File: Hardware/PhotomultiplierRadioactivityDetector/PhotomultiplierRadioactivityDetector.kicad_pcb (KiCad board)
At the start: 2 copper layers, 100 x 100 mm, 102 parts, among them J13 Conn_01x02_Female, J14 Conn_01x04, J15 Conn_02x05_Counter_Clockwise, Q1 2N7002, Q2 Q_NPN_BEC, Q3 Q_NMOS_GDS, U1 TL074, U2 TL074, U3 MCP3425A0T-ECH, U4 LM3488, U5 STM8S003F3P

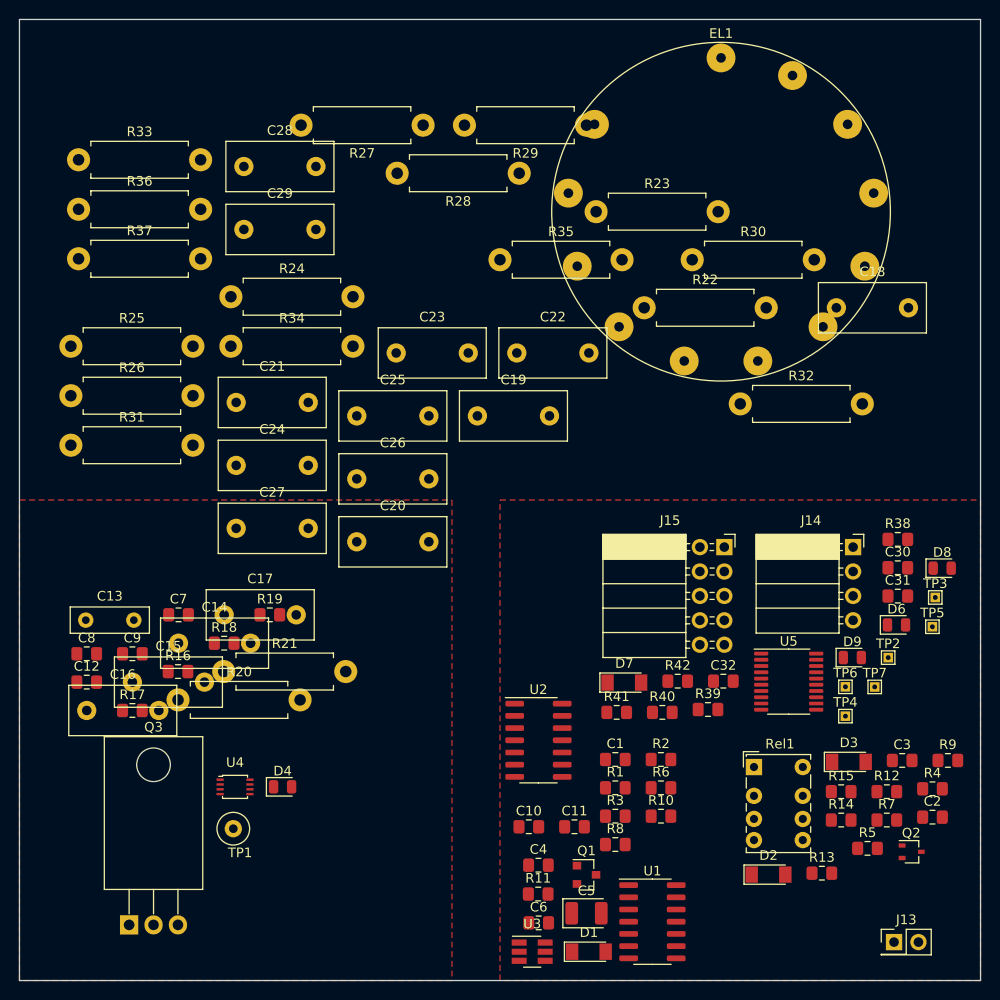
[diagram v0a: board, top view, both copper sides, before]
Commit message: draft of amplifier
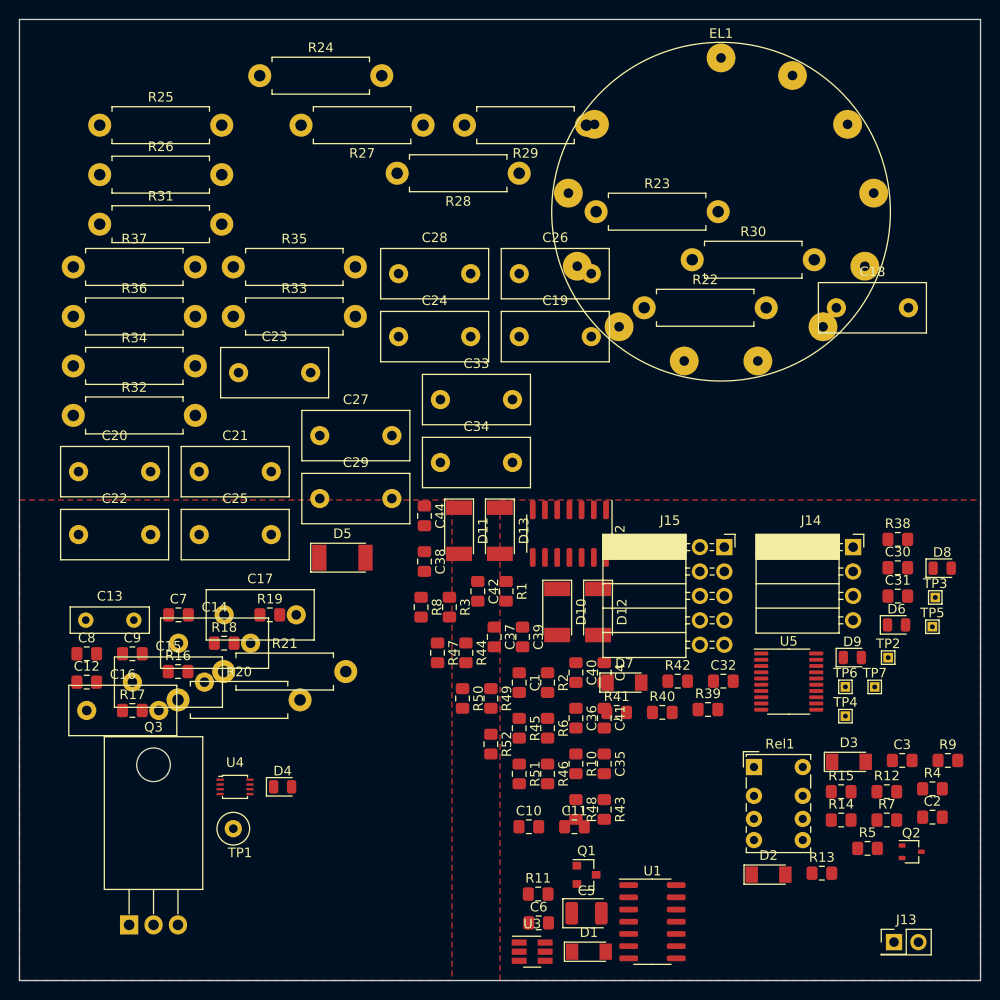
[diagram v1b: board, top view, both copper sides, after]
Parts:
- added C33: 10n/3kV, Capacitor_THT:C_Disc_D11.0mm_W5.0mm_P7.50mm, F.Cu at (68.8, 129.6)
- added C34: 10n/3kV, Capacitor_THT:C_Disc_D11.0mm_W5.0mm_P7.50mm, F.Cu at (68.8, 136.1)
- added C35: 2p2, Capacitor_SMD:C_0805_2012Metric_Pad1.15x1.40mm_HandSolder, F.Cu at (85.8, 167.4)
- added C36: 2p2, Capacitor_SMD:C_0805_2012Metric_Pad1.15x1.40mm_HandSolder, F.Cu at (82.9, 162.7)
- added C37: 1n, Capacitor_SMD:C_0805_2012Metric_Pad1.15x1.40mm_HandSolder, F.Cu at (74.4, 154.2)
- added C38: 1n, Capacitor_SMD:C_0805_2012Metric_Pad1.15x1.40mm_HandSolder, F.Cu at (67.1, 146.4)
- added C39: 100n, Capacitor_SMD:C_0805_2012Metric_Pad1.15x1.40mm_HandSolder, F.Cu at (77.3, 154.2)
- added C40: 100n, Capacitor_SMD:C_0805_2012Metric_Pad1.15x1.40mm_HandSolder, F.Cu at (82.9, 157.9)
- added C41: 4p7+2p2, Capacitor_SMD:C_0805_2012Metric_Pad1.15x1.40mm_HandSolder, F.Cu at (85.8, 162.7)
- added C42: 4p7+2p2, Capacitor_SMD:C_0805_2012Metric_Pad1.15x1.40mm_HandSolder, F.Cu at (72.7, 149.5)
- added C44: 100n, Capacitor_SMD:C_0805_2012Metric_Pad1.15x1.40mm_HandSolder, F.Cu at (67.1, 141.7)
- added D10: 1n148, Diode_SMD:D_MELF, F.Cu at (81.0, 151.7)
- added D11: 1n148, Diode_SMD:D_MELF, F.Cu at (70.7, 143.2)
- added D12: 1n148, Diode_SMD:D_MELF, F.Cu at (85.2, 151.7)
- added D13: 1n148, Diode_SMD:D_MELF, F.Cu at (75.0, 143.2)
- added D5: D, Diode_SMD:D_MELF, F.Cu at (58.6, 146.0)
- added R43: 10G, Resistor_SMD:R_0805_2012Metric_Pad1.15x1.40mm_HandSolder, F.Cu at (85.8, 172.2)
- added R44: 10G, Resistor_SMD:R_0805_2012Metric_Pad1.15x1.40mm_HandSolder, F.Cu at (71.5, 155.9)
- added R45: 10k, Resistor_SMD:R_0805_2012Metric_Pad1.15x1.40mm_HandSolder, F.Cu at (77.0, 163.8)
- added R46: 10k, Resistor_SMD:R_0805_2012Metric_Pad1.15x1.40mm_HandSolder, F.Cu at (80.0, 168.5)
- added R47: 10k, Resistor_SMD:R_0805_2012Metric_Pad1.15x1.40mm_HandSolder, F.Cu at (68.5, 155.9)
- added R48: 10k, Resistor_SMD:R_0805_2012Metric_Pad1.15x1.40mm_HandSolder, F.Cu at (82.9, 172.2)
- added R49: 10k, Resistor_SMD:R_0805_2012Metric_Pad1.15x1.40mm_HandSolder, F.Cu at (74.0, 160.7)
- added R50: 10k, Resistor_SMD:R_0805_2012Metric_Pad1.15x1.40mm_HandSolder, F.Cu at (71.1, 160.7)
- added R51: 10M, Resistor_SMD:R_0805_2012Metric_Pad1.15x1.40mm_HandSolder, F.Cu at (77.0, 168.5)
- added R52: 10M, Resistor_SMD:R_0805_2012Metric_Pad1.15x1.40mm_HandSolder, F.Cu at (74.0, 165.4)
- C1: value 10n -> 100n
- R10, R8: value 10k -> 0R
- moved R32 69.4 mm to (30.6, 131.2)
- moved C22 49.4 mm to (31.1, 143.6)
- moved R8 31.9 mm to (66.8, 151.2), turned to 270 degrees
- moved C20 29.9 mm to (31.1, 137.1)
- moved C29 29.1 mm to (56.2, 139.8)
- moved R3 27.8 mm to (69.7, 151.2), turned to 270 degrees
- moved R35 27.8 mm to (47.2, 115.8)
- moved C26 27.2 mm to (77.0, 116.5)
- moved R1 23.4 mm to (75.6, 149.5), turned to 270 degrees
- moved R31 23.2 mm to (33.4, 111.3)
- moved R24 23.2 mm to (50.0, 95.8)
- moved R25 23.2 mm to (33.4, 101.0)
- moved R26 23.2 mm to (33.4, 106.2)
- moved R33 22.9 mm to (47.2, 120.9)
- moved U2 21.7 mm to (82.2, 143.5), turned to 270 degrees
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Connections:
- C1 pad 1: ANODE_OUTPUT -> Net-(C1-Pad1)
- C1 pad 2: Net-(C1-Pad2) -> GND
- C10 pad 2: ANODE_OUTPUT -> GND
- C11 pad 2: ANODE_OUTPUT -> GND
- C12 pad 2: ANODE_OUTPUT -> GND
- C13 pad 2: ANODE_OUTPUT -> GND
- C14 pad 1: ANODE_OUTPUT -> GND
- C15 pad 1: ANODE_OUTPUT -> GND
- C16 pad 1: ANODE_OUTPUT -> GND
- C17 pad 1: ANODE_OUTPUT -> GND
- C18 pad 1: Net-(C18-Pad1) -> GND
- C18 pad 2: ANODE_OUTPUT -> Net-(C18-Pad2)
- C20 pad 2: ANODE_OUTPUT -> DYNOE_OUTPUT
- C21 pad 2: ANODE_OUTPUT -> Net-(C18-Pad2)
- C22 pad 2: ANODE_OUTPUT -> Net-(C21-Pad1)
- C23 pad 2: ANODE_OUTPUT -> Net-(C22-Pad1)
- C24 pad 2: ANODE_OUTPUT -> Net-(C23-Pad1)
- C25 pad 1: Net-(C25-Pad1) -> GND
- C25 pad 2: ANODE_OUTPUT -> Net-(C24-Pad1)
- C26 pad 2: ANODE_OUTPUT -> Net-(C18-Pad2)
- C27 pad 2: ANODE_OUTPUT -> Net-(C26-Pad1)
- C28 pad 2: Net-(C28-Pad2) -> Net-(C27-Pad1)
- C29 pad 1: (no net) -> Net-(C29-Pad1)
- C29 pad 2: Net-(C29-Pad2) -> Net-(C28-Pad1)
- C3 pad 1: ANODE_OUTPUT -> GND
- C30 pad 1: ANODE_OUTPUT -> GND
- C31 pad 1: ANODE_OUTPUT -> GND
- C32 pad 1: ANODE_OUTPUT -> GND
- C4 pad 1: ANODE_OUTPUT -> Net-(C4-Pad1)
- C4 pad 2: VCC_5V -> GND
- C5 pad 2: ANODE_OUTPUT -> GND
- C6 pad 1: ANODE_OUTPUT -> GND
- C7 pad 1: ANODE_OUTPUT -> GND
- C8 pad 1: ANODE_OUTPUT -> GND
- C9 pad 1: ANODE_OUTPUT -> GND
- D6 pad 1: ANODE_OUTPUT -> GND
- D8 pad 1: ANODE_OUTPUT -> GND
- D9 pad 1: ANODE_OUTPUT -> GND
- EL1 pad 1: Net-(C18-Pad1) -> Net-(C18-Pad2)
- EL1 pad 10: Net-(EL1-Pad10) -> Net-(C33-Pad1)
- EL1 pad 11: Net-(C28-Pad1) -> Net-(EL1-Pad11)
- EL1 pad 12: Net-(EL1-Pad12) -> GND
- EL1 pad 2: Net-(C19-Pad1) -> Net-(C26-Pad1)
- EL1 pad 3: Net-(C20-Pad1) -> Net-(C21-Pad1)
- EL1 pad 4: Net-(C21-Pad1) -> Net-(C27-Pad1)
- EL1 pad 6: Net-(C23-Pad1) -> Net-(C28-Pad1)
- EL1 pad 7: Net-(C24-Pad1) -> Net-(C23-Pad1)
- EL1 pad 8: Net-(C25-Pad1) -> Net-(C29-Pad1)
- EL1 pad 9: Net-(C26-Pad1) -> Net-(C24-Pad1)
- J13 pad 1: ANODE_OUTPUT -> GND
- J14 pad 4: ANODE_OUTPUT -> GND
- J15 pad 3: ANODE_OUTPUT -> GND
- Q1 pad 2: ANODE_OUTPUT -> GND
- Q2 pad 2: ANODE_OUTPUT -> GND
- R1 pad 1: VCC_5V -> VCC
- R1 pad 2: Net-(C1-Pad2) -> Net-(C1-Pad1)
- R10 pad 1: Net-(R10-Pad1) -> DYNOE_OUTPUT
- R10 pad 2: Net-(R10-Pad2) -> Net-(C36-Pad2)
- R13 pad 2: ANODE_OUTPUT -> GND
- R15 pad 2: ANODE_OUTPUT -> GND
- R16 pad 2: ANODE_OUTPUT -> GND
- R18 pad 2: ANODE_OUTPUT -> GND
- R19 pad 2: ANODE_OUTPUT -> GND
- R2 pad 1: Net-(C1-Pad2) -> Net-(C1-Pad1)
- R2 pad 2: ANODE_OUTPUT -> GND
- R21 pad 2: ANODE_OUTPUT -> GND
- R22 pad 2: Net-(C18-Pad1) -> Net-(C18-Pad2)
- R23 pad 1: Net-(C19-Pad1) -> Net-(C26-Pad1)
- R23 pad 2: Net-(C18-Pad1) -> Net-(C18-Pad2)
- R24 pad 1: Net-(C20-Pad1) -> Net-(C21-Pad1)
- R24 pad 2: Net-(C19-Pad1) -> Net-(C26-Pad1)
- R25 pad 1: Net-(C21-Pad1) -> Net-(C27-Pad1)
- R25 pad 2: Net-(C20-Pad1) -> Net-(C21-Pad1)
- R26 pad 2: Net-(C21-Pad1) -> Net-(C27-Pad1)
- R27 pad 1: Net-(C23-Pad1) -> Net-(C28-Pad1)
- R28 pad 1: Net-(C24-Pad1) -> Net-(C23-Pad1)
- R28 pad 2: Net-(C23-Pad1) -> Net-(C28-Pad1)
- R29 pad 1: Net-(C25-Pad1) -> Net-(C29-Pad1)
- R29 pad 2: Net-(C24-Pad1) -> Net-(C23-Pad1)
- R3 pad 1: (no net) -> VCC
- R3 pad 2: Net-(R3-Pad2) -> Net-(C4-Pad1)
- R30 pad 1: Net-(C26-Pad1) -> Net-(C24-Pad1)
- R30 pad 2: Net-(C25-Pad1) -> Net-(C29-Pad1)
- R31 pad 1: Net-(C27-Pad1) -> Net-(C33-Pad1)
- R31 pad 2: Net-(C26-Pad1) -> Net-(C24-Pad1)
- R32 pad 1: Net-(C29-Pad2) -> ANODE_OUTPUT
- R32 pad 2: Net-(EL1-Pad10) -> GND
- R33 pad 1: Net-(C27-Pad1) -> DYNOE_OUTPUT
- R33 pad 2: Net-(C29-Pad2) -> GND
- R34 pad 1: Net-(C28-Pad2) -> Net-(C18-Pad2)
- R34 pad 2: Net-(C27-Pad1) -> Net-(C19-Pad1)
- R35 pad 1: Net-(C28-Pad1) -> Net-(C26-Pad1)
- R35 pad 2: Net-(C28-Pad2) -> Net-(C20-Pad1)
- R36 pad 1: ANODE_OUTPUT -> Net-(EL1-Pad11)
- R36 pad 2: Net-(C28-Pad1) -> Net-(C33-Pad1)
- R37 pad 1: ANODE_OUTPUT -> GND
- R37 pad 2: Net-(EL1-Pad12) -> Net-(EL1-Pad11)
- R6 pad 1: Net-(R3-Pad2) -> Net-(C4-Pad1)
- R6 pad 2: Net-(R6-Pad2) -> GND
- R7 pad 2: ANODE_OUTPUT -> GND
- R8 pad 1: Net-(R6-Pad2) -> ANODE_OUTPUT
- R8 pad 2: Net-(R10-Pad1) -> Net-(C35-Pad2)
- R9 pad 2: ANODE_OUTPUT -> GND
- U1 pad 10: Net-(C1-Pad2) -> Net-(C4-Pad1)
- U1 pad 11: (no net) -> GND
- U1 pad 12: Net-(C1-Pad2) -> Net-(C40-Pad1)
- U1 pad 13: Net-(R10-Pad1) -> Net-(C42-Pad2)
- U1 pad 14: Net-(R10-Pad2) -> Net-(C42-Pad1)
- U1 pad 4: (no net) -> Net-(C44-Pad1)
- U1 pad 8: Net-(R6-Pad2) -> Net-(C36-Pad1)
- U1 pad 9: Net-(R3-Pad2) -> DYNOE_OUTPUT
- U2 pad 1: (no net) -> Net-(C35-Pad1)
- U2 pad 11: ANODE_OUTPUT -> (no net)
- U2 pad 2: (no net) -> ANODE_OUTPUT
- U2 pad 3: (no net) -> Net-(C1-Pad1)
- U2 pad 4: VCC_5V -> (no net)
- U2 pad 5: (no net) -> Net-(C39-Pad1)
- U2 pad 6: (no net) -> Net-(C41-Pad2)
- U2 pad 7: (no net) -> Net-(C41-Pad1)
- U3 pad 2: ANODE_OUTPUT -> GND
- U4 pad 4: ANODE_OUTPUT -> GND
- U5 pad 7: ANODE_OUTPUT -> GND
